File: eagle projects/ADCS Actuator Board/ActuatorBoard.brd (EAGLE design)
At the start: 91 x 91 mm, 278 parts, among them J19 TE_1-84953-1, J20 TE_1-84953-1, J21 TE_1-84953-1, U10 DRV10970_MOTOR_DRIVERDRV10970, U12 DRV10970_MOTOR_DRIVERDRV10970, U13 ADS7841E_2K5, U15 TLV9051IDCKR, U19 TLV9051IDCKR, U2 ADS7841E_2K5, U21 TLV9051IDCKR, U23 TLV9051IDCKR, U24 TLV9051IDCKR, U25 ADS7841E_2K5, U26 TLV9051IDCKR, U27 ADS7841E_2K5, U28 TLV9051IDCKR, U29 TLV9051IDCKR, U3 ADS7841E_2K5, U30 TLV9051IDCKR, U31 TLV9051IDCKR, U32 TLV9051IDCKR, U34 TVS991, U35 BD6210F-E2, U38 TVS991, U39 BD6210F-E2, U4 ADS7841E_2K5, U5 TVS991, U6 TLV9051IDCKR, U7 DRV10970_MOTOR_DRIVERDRV10970, U9 BD6210F-E2

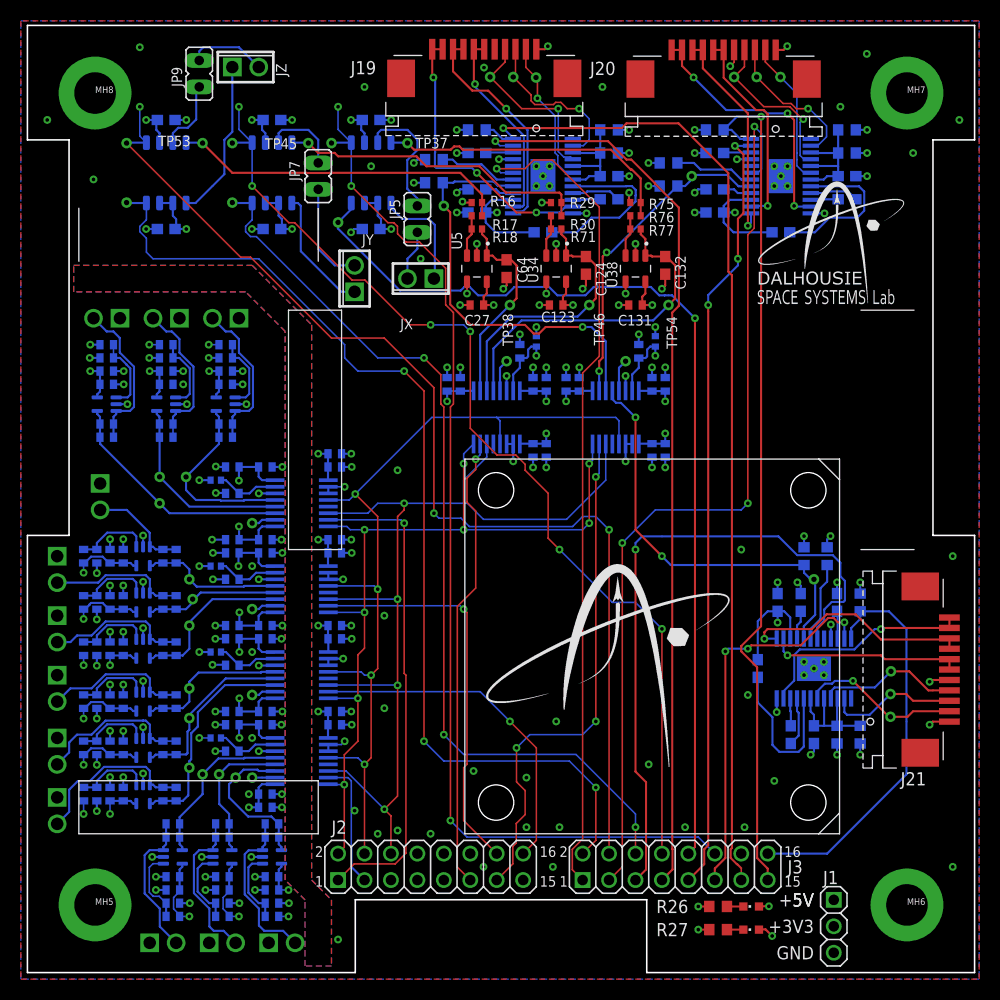
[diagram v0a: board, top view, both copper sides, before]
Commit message: Slight layout tweaks
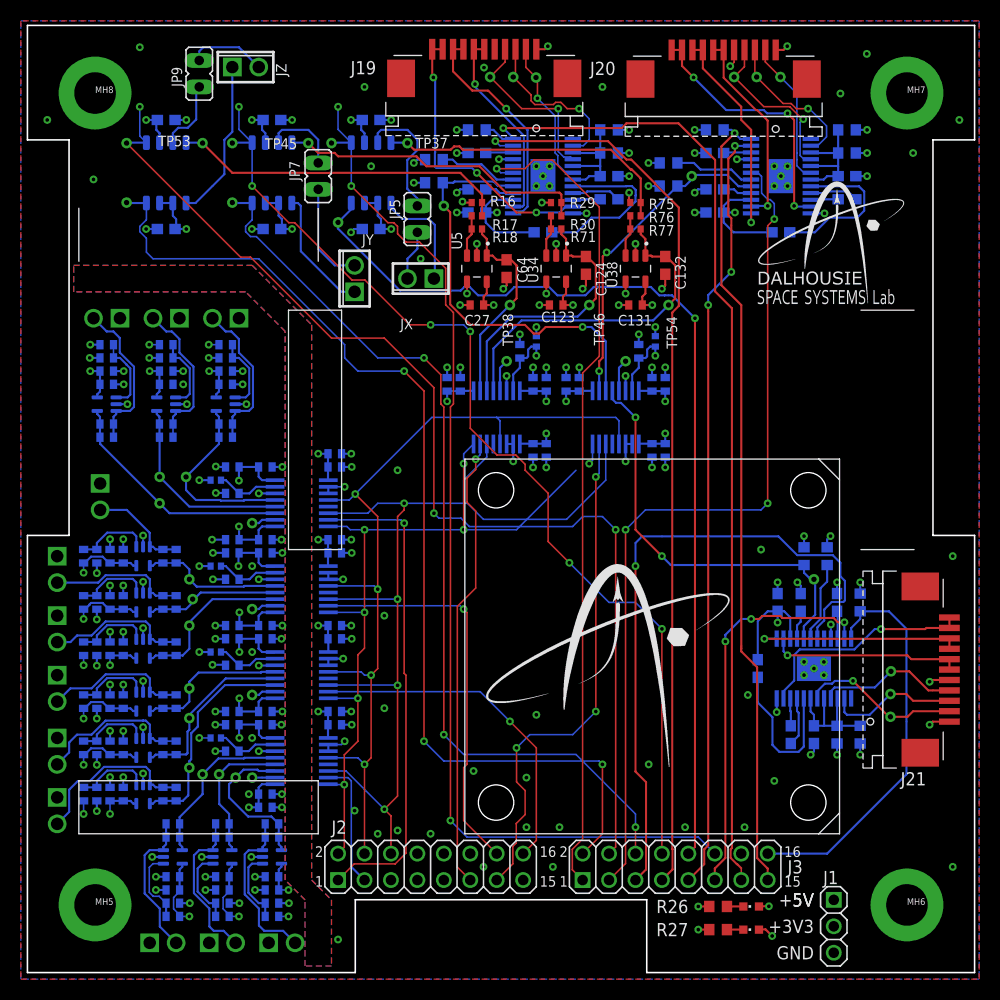
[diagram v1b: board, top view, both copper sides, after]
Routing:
- net RW_Y_SPEED_CTRL: track 88.5 -> 82.5 mm
- net RW_Y_OUTFG: track 82.3 -> 77.4 mm
- net UCB0_SPI_CLK: track 81.9 -> 77.0 mm, vias 8 -> 7
- net Z_PHASE_B: track 22.4 -> 20.0 mm
- net MAG_Z_FIN: track 99.0 -> 101.2 mm
- net RW_Z_DIR: track 36.9 -> 38.0 mm
- net MAG_Z_RIN: track 106.4 -> 107.3 mm
- net Y_PHASE_B: track 21.0 -> 20.4 mm
- net !CS!_CUR_SENSE_RW: track 49.6 -> 49.1 mm
